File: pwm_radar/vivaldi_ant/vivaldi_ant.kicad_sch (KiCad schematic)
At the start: 2 parts, among them J1 Conn_Coaxial

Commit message: added ant
added antenna
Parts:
- J1: footprint (none) -> Connector_Coaxial:SMA_Amphenol_132289_EdgeMount
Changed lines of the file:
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@@
 			)
 		)
-		(property "Footprint" ""
+		(property "Footprint" "Connector_Coaxial:SMA_Amphenol_132289_EdgeMount"
 			(at 105.41 102.87 0)
 			(effects

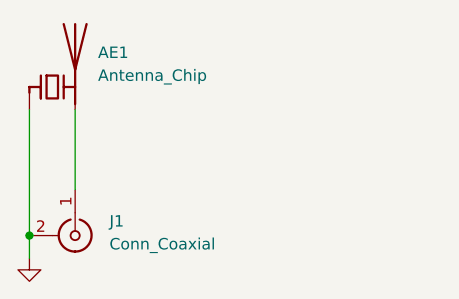
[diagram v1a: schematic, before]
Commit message: fixing some final touches
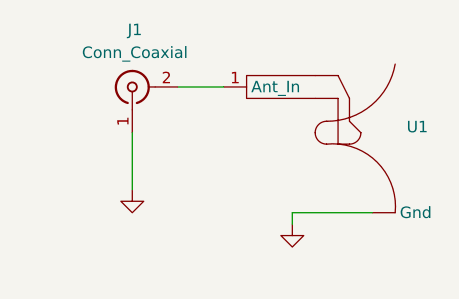
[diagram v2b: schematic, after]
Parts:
- removed AE1: Antenna_Chip, symbol Device:Antenna_Chip
- added U1: ~, RF_Antenna:Vivaldi Antenna 10 to 24 GHz, symbol antenna_lib:Vivaldi_Antenna_10_24
- J1: footprint Connector_Coaxial:SMA_Amphenol_132289_EdgeMount -> (none)
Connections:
- net GND: now also J1.1 (In), U1. (Gnd); no longer J1.2 (Ext)
- new net: J1.2 (Ext), U1.1 (Ant_In)
